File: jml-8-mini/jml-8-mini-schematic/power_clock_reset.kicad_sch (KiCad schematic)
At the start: 21 parts, among them J1 BarrelJack, SW1 SW_Push, SW2 SW_Push_DPDT, U10 74LS74, U11 NE555P, U6 74LS04, X1 8MHz, X2 2.4576MHz

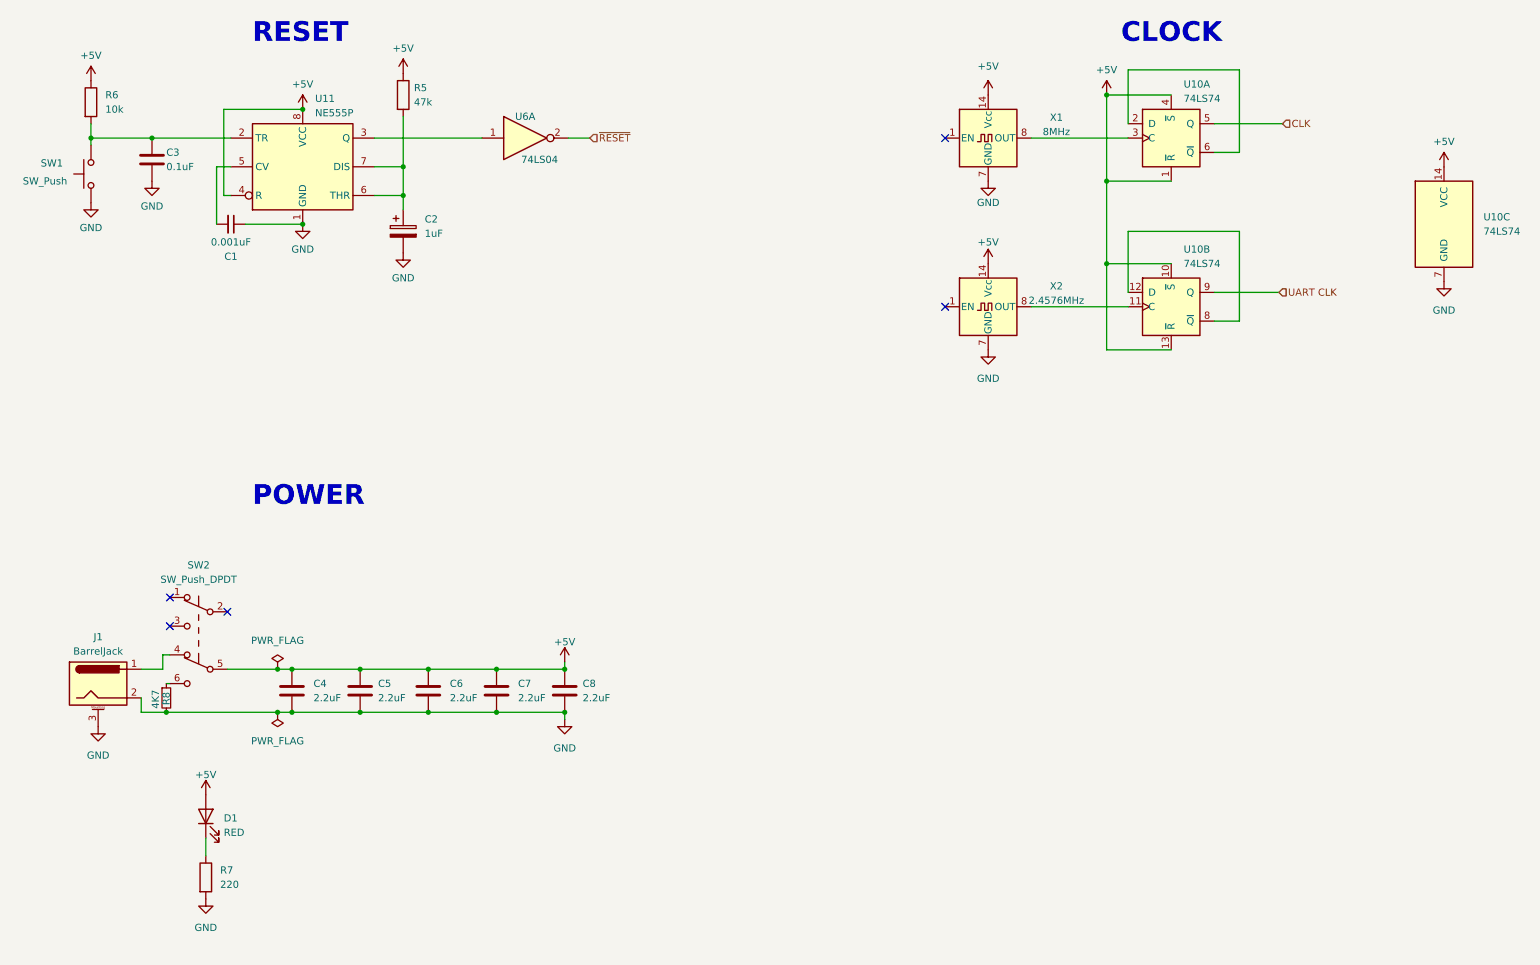
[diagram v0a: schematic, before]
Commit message: lots of updates to schematic to make pcb routing easier, start on pcb design
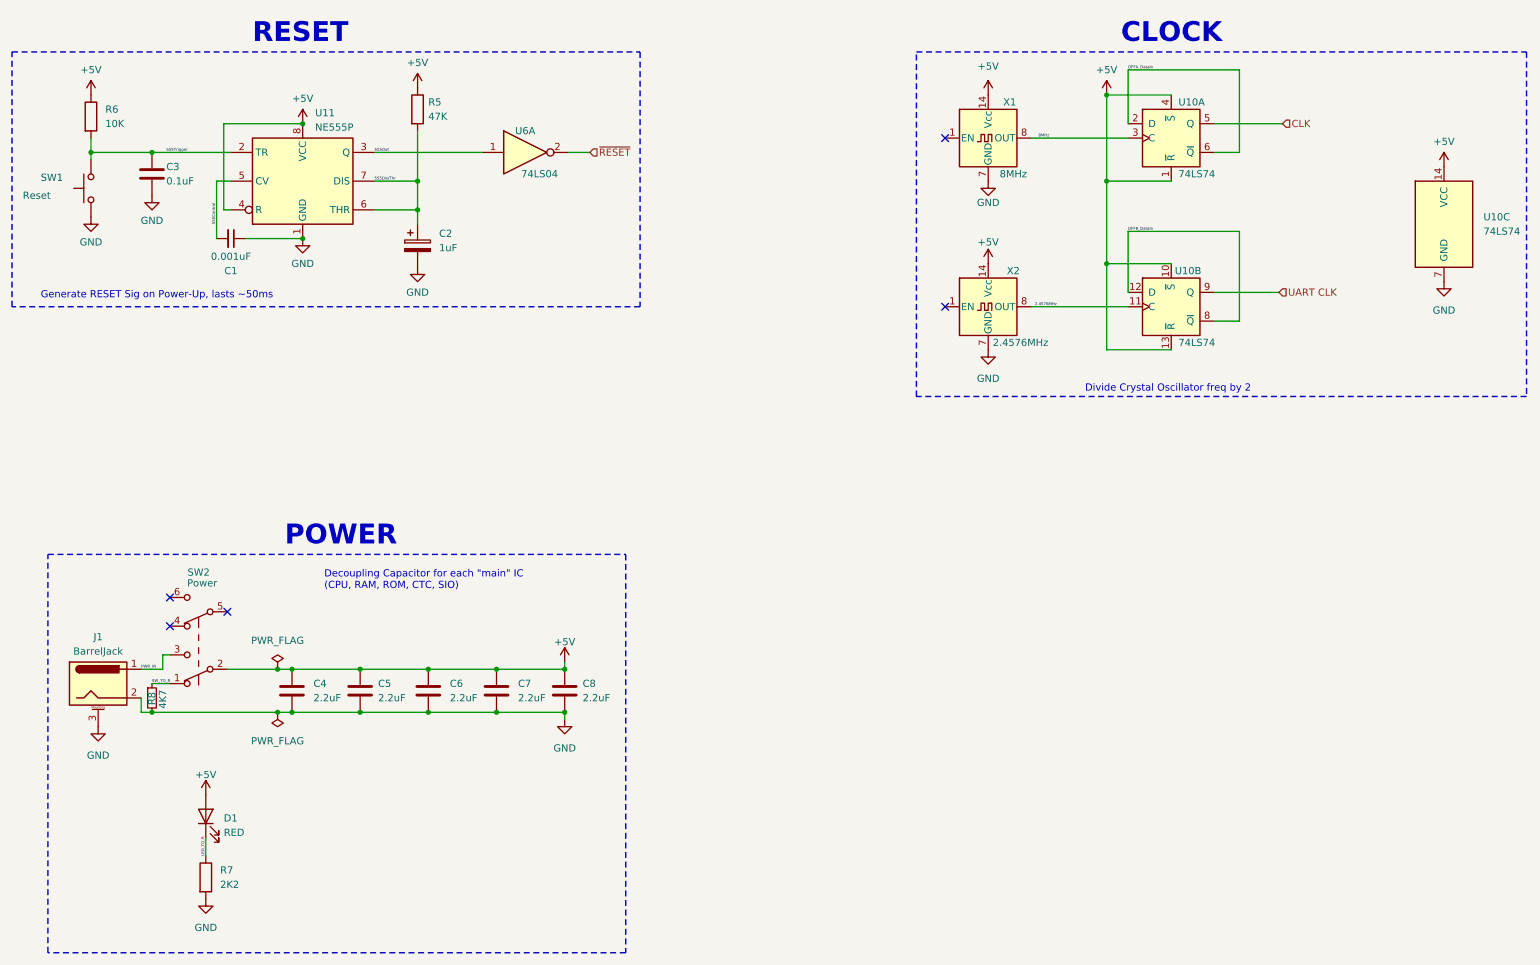
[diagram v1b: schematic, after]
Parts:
- R5: value 47k -> 47K
- R6: value 10k -> 10K
- R7: value 220 -> 2K2
- SW1: value SW_Push -> Reset
- SW2: value SW_Push_DPDT -> Power
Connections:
- net +5V: now also SW2.2 (B); no longer SW2.5 (B)
- net 2.4576MHz: now reaches U10.11 (C), X2.8 (OUT)
- net DFFB_DataIn: now reaches U10.12 (D), U10.8 (~{Q})
- net 555Trigger: now reaches C3.1, R6.2, SW1.2, U11.2 (TR)
- net LED_TO_R: now reaches D1.1 (K), R7.1
- net at SW2.6 (C): no longer R8.1
- net at SW2.4 (A): no longer J1.1
- net 555Dis/Thr: now reaches C2.1, R5.2, U11.6 (THR), U11.7 (DIS)
- net DFFA_DataIn: now reaches U10.2 (D), U10.6 (~{Q})
- net 8MHz: now reaches U10.3 (C), X1.8 (OUT)
- net SW_TO_R: now reaches SW2.1 (A)
- net SW_TO_R: now also R8.1
- net PWR_IN: now reaches SW2.3 (C)
- net PWR_IN: now also J1.1
- net 555Out: now reaches U11.3 (Q), U6.1
- net 555Control: now reaches C1.2, U11.5 (CV)
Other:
- note added: "Decoupling Capacitor for each "main" IC (CPU, RAM, ROM, CTC, SIO)"
- note added: "Divide Crystal Oscillator freq by 2"
- note added: "Generate RESET Sig on Power-Up, lasts ~50ms"
- moved on the sheet: C1, C2, C3, R5, R6, R8, SW1, SW2, U11, U6A
